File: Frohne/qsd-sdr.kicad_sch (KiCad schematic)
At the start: 50 parts, among them J11 SDR ANT, J12 SDR Out, U5 OPA1612AxD, U7 SN74CBT3253, U8 OPA1612AxD

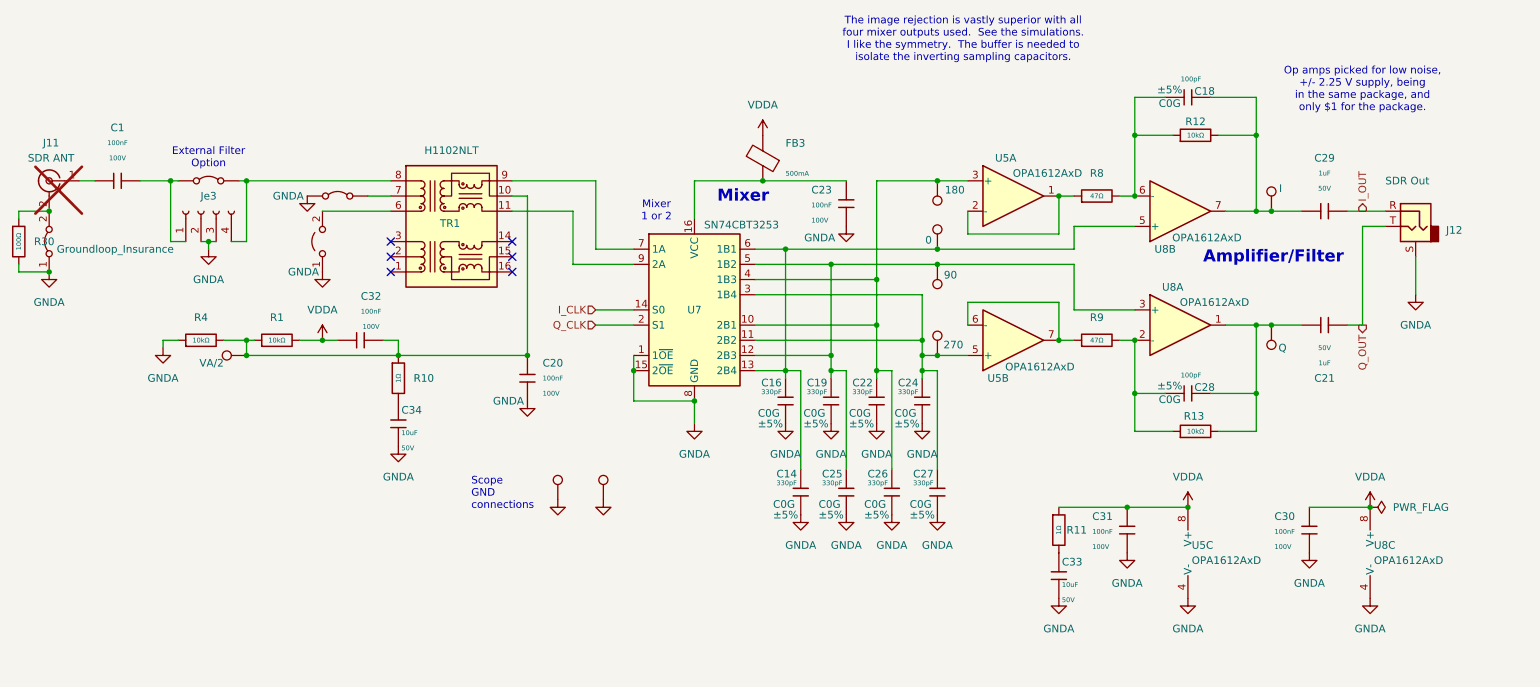
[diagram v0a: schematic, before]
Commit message: Added DAC
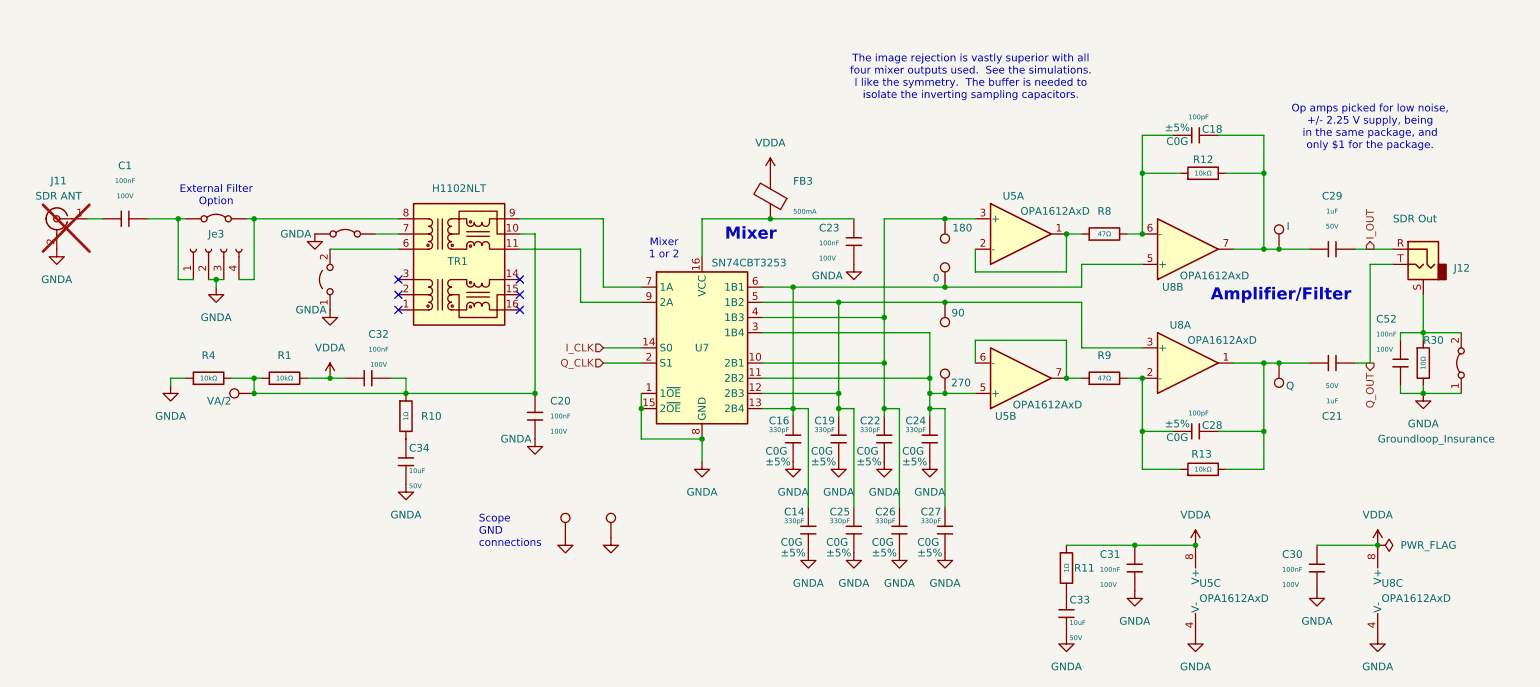
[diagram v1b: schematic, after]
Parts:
- removed R30: 100Ω, PCM_JLCPCB:R_0805, symbol PCM_JLCPCB-Resistors:0805,100Ω
- removed e2: Groundloop_Insurance, Jumper:SolderJumper-2_P1.3mm_Bridged_RoundedPad1.0x1.5mm, symbol Jumper:Jumper_2_Bridged
- added C52: 100nF, PCM_JLCPCB:C_0805, symbol PCM_JLCPCB-Capacitors:0805,100nF
- added R30: 10Ω, PCM_JLCPCB:R_0603, symbol PCM_JLCPCB-Resistors:0603,10Ω
- added e5: Groundloop_Insurance, Jumper:SolderJumper-2_P1.3mm_Bridged_RoundedPad1.0x1.5mm, symbol Jumper:Jumper_2_Bridged
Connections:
- net GNDA: now also J11.2 (Ext), C52.1, R30.2, e5.1 (A); no longer J12.S
- new net: C52.2, J12.S, R30.1, e5.2 (B)
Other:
- moved on the sheet: C1, C14, C16, C18, C19, C20, C21, C22, C23, C24, C25, C26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
